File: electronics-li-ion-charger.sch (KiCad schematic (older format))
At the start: 16 parts

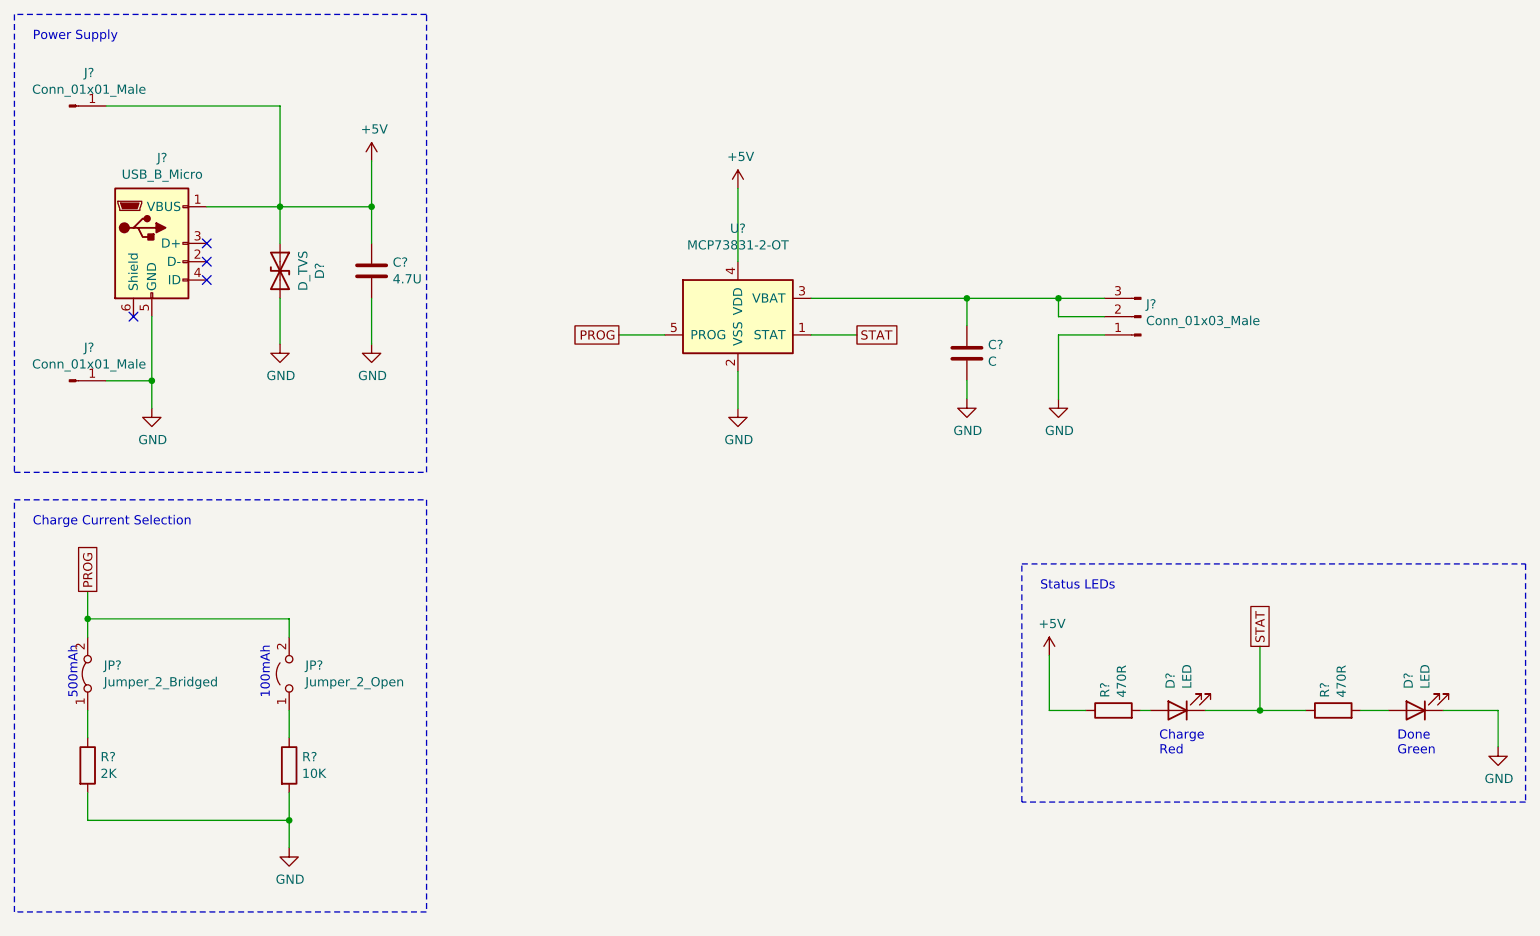
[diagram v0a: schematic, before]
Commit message: Complete schematic.
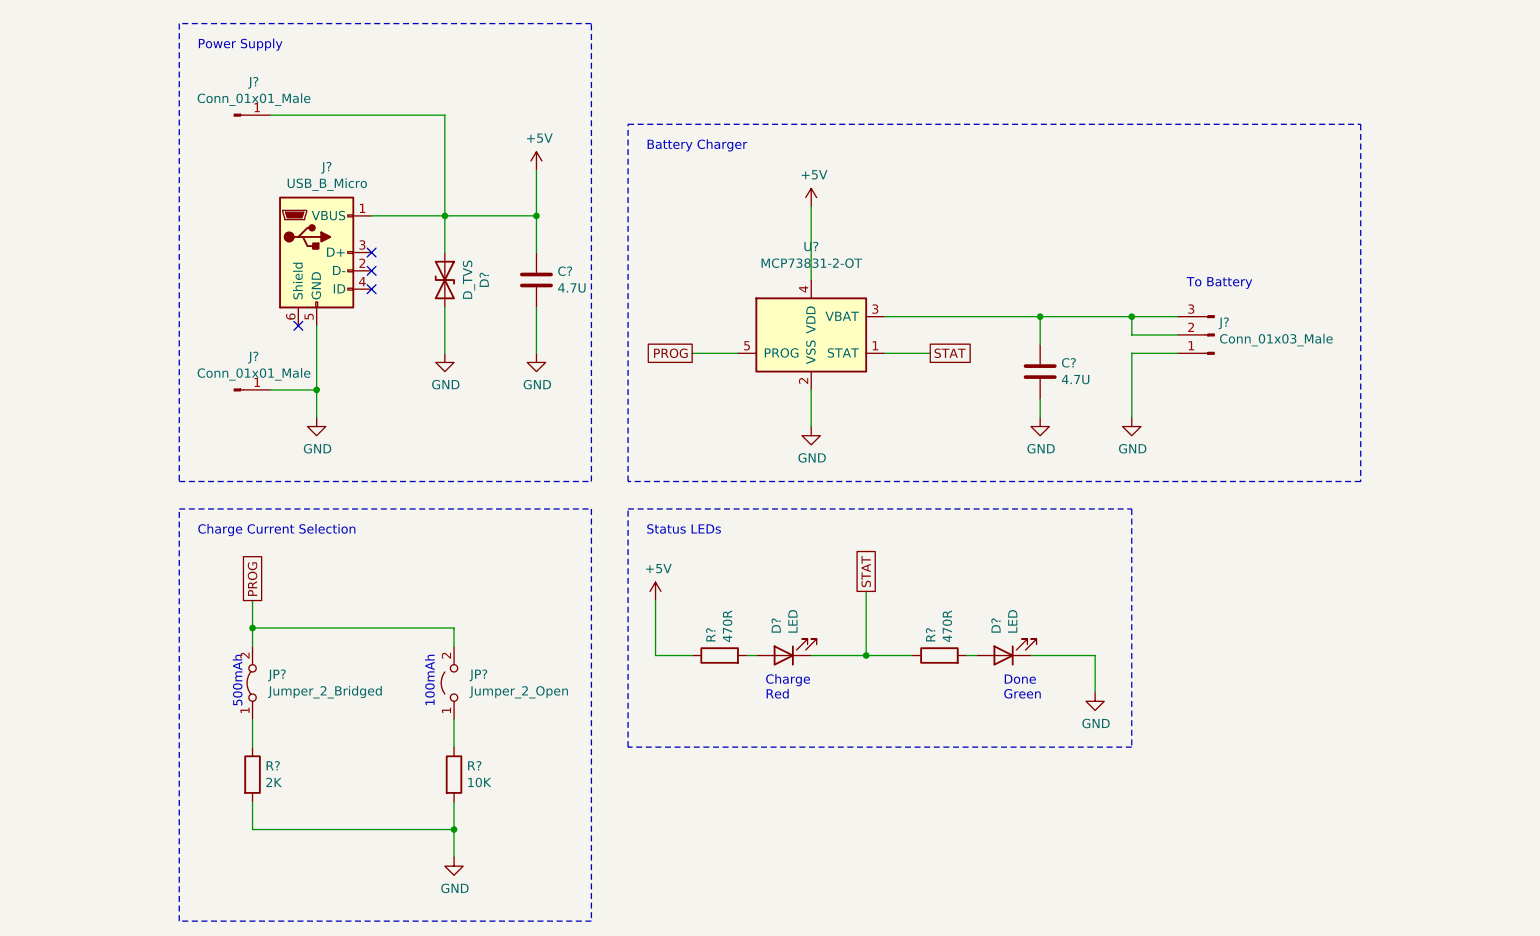
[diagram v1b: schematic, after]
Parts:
- C?: value C -> 4.7U; footprint (none) -> Capacitor_SMD:C_1206_3216Metric_Pad1.33x1.80mm_HandSolder
- J?: footprint (none) -> Connector_PinHeader_2.54mm:PinHeader_1x03_P2.54mm_Vertical
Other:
- note added: "Battery Charger"
- note added: "To Battery"
- moved on the sheet: C?, D?, J?, JP?, R?, U?
